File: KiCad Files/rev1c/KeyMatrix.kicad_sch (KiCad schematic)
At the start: 105 parts, among them SW1 SW_Push, SW10 SW_Push, SW11 SW_Push, SW12 SW_Push, SW13 SW_Push, SW14 SW_Push, SW15 SW_Push, SW16 SW_Push, SW17 SW_Push, SW18 SW_Push, SW19 SW_Push, SW2 SW_Push, SW20 SW_Push, SW21 SW_Push, SW22 SW_Push, SW23 SW_Push, SW24 SW_Push, SW25 SW_Push, SW26 SW_Push, SW27 SW_Push, SW28 SW_Push, SW29 SW_Push, SW3 SW_Push, SW30 SW_Push, SW31 SW_Push, SW32 SW_Push, SW33 SW_Push, SW34 SW_Push, SW35 SW_Push, SW36 SW_Push, SW37 SW_Push, SW38 SW_Push, SW39 SW_Push, SW4 SW_Push, SW40 SW_Push, SW41 SW_Push, SW42 SW_Push, SW43 SW_Push, SW44 SW_Push, SW45 SW_Push, SW46 SW_Push, SW47 SW_Push, SW48 SW_Push, SW49 SW_Push, SW5 SW_Push, SW50 SW_Push, SW51 SW_Push, SW52 SW_Push, SW53 SW_Push, SW54 SW_Push, SW55 SW_Push, SW56 SW_Push, SW57 SW_Push, SW58 SW_Push, SW59 SW_Push, SW6 SW_Push, SW60 SW_Push, SW61 SW_Push, SW62 SW_Push, SW63 SW_Push, SW64 SW_Push, SW65 SW_Push, SW66 SW_Push, SW67 SW_Push, SW68 SW_Push, SW69 SW_Push, SW7 SW_Push, SW70 SW_Push, SW71 SW_Push, SW72 SW_Push, SW8 SW_Push, SW9 SW_Push

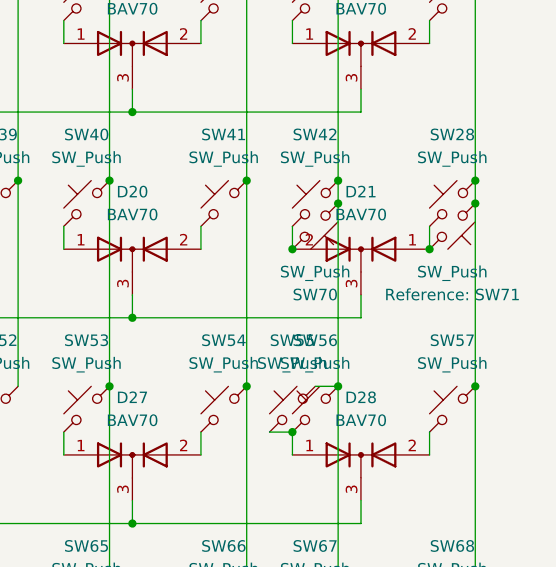
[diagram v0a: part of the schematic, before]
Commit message: update on pcb
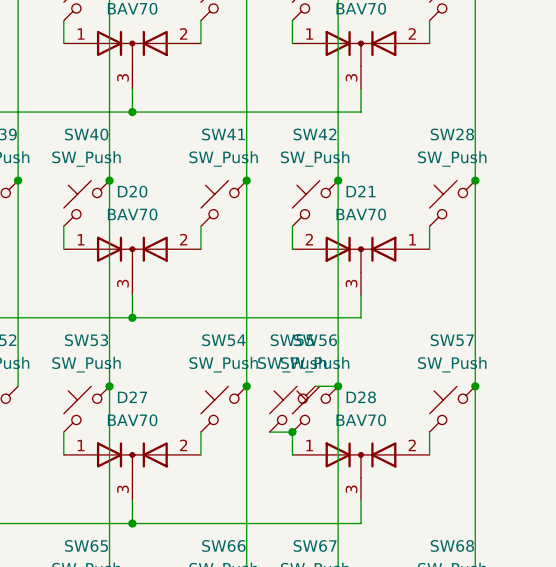
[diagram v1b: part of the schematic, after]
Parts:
- removed SW70: SW_Push, PCM_Switch_Keyboard_Hotswap_Kailh:SW_Hotswap_Kailh_MX_Plated_1.50u, symbol Switch:SW_Push_45deg
- removed SW71: SW_Push, PCM_Switch_Keyboard_Hotswap_Kailh:SW_Hotswap_Kailh_MX_Plated_2.25u, symbol Switch:SW_Push_45deg
